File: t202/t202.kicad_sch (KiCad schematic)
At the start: 7 parts, among them J1 Conn_02x04_Counter_Clockwise, SW1 SW_Push, U1 ATtiny202-SS

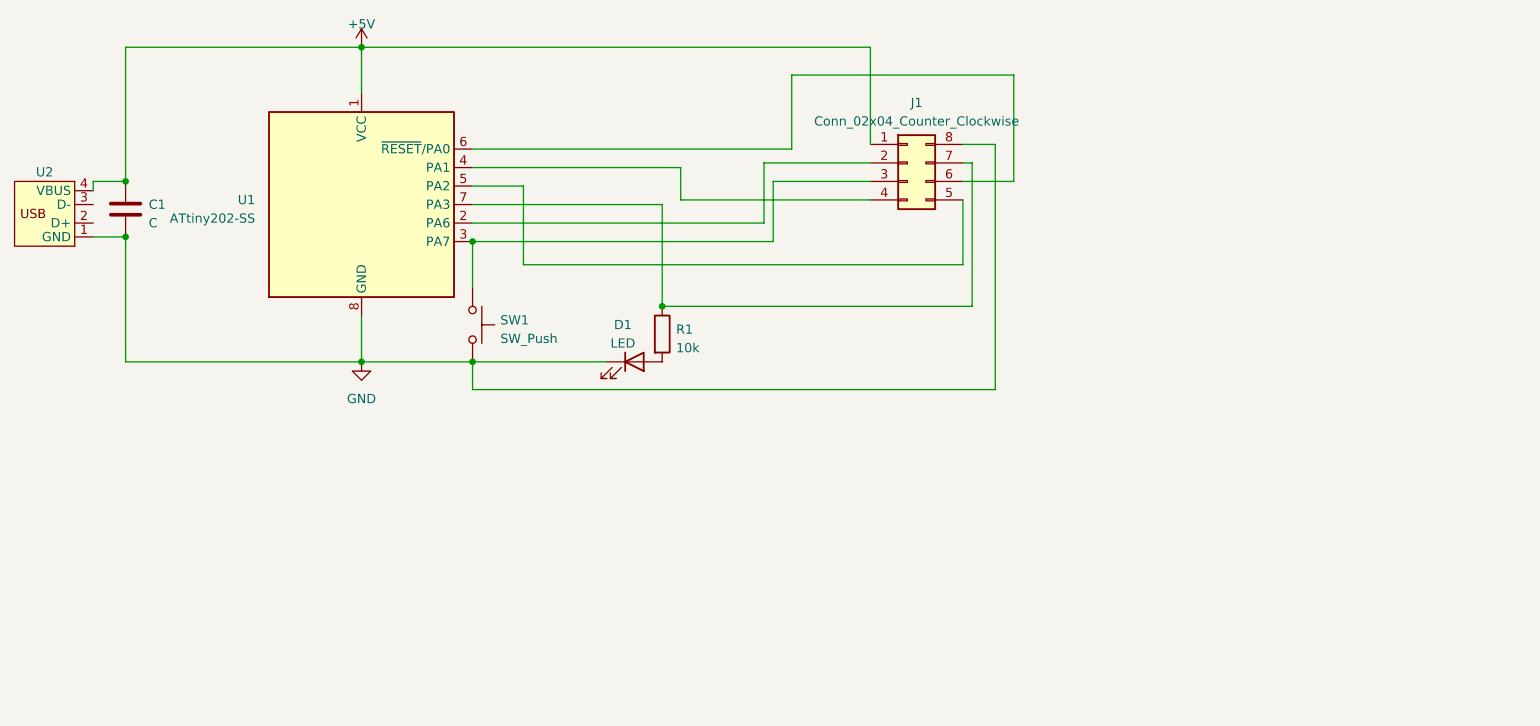
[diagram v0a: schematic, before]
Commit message: -
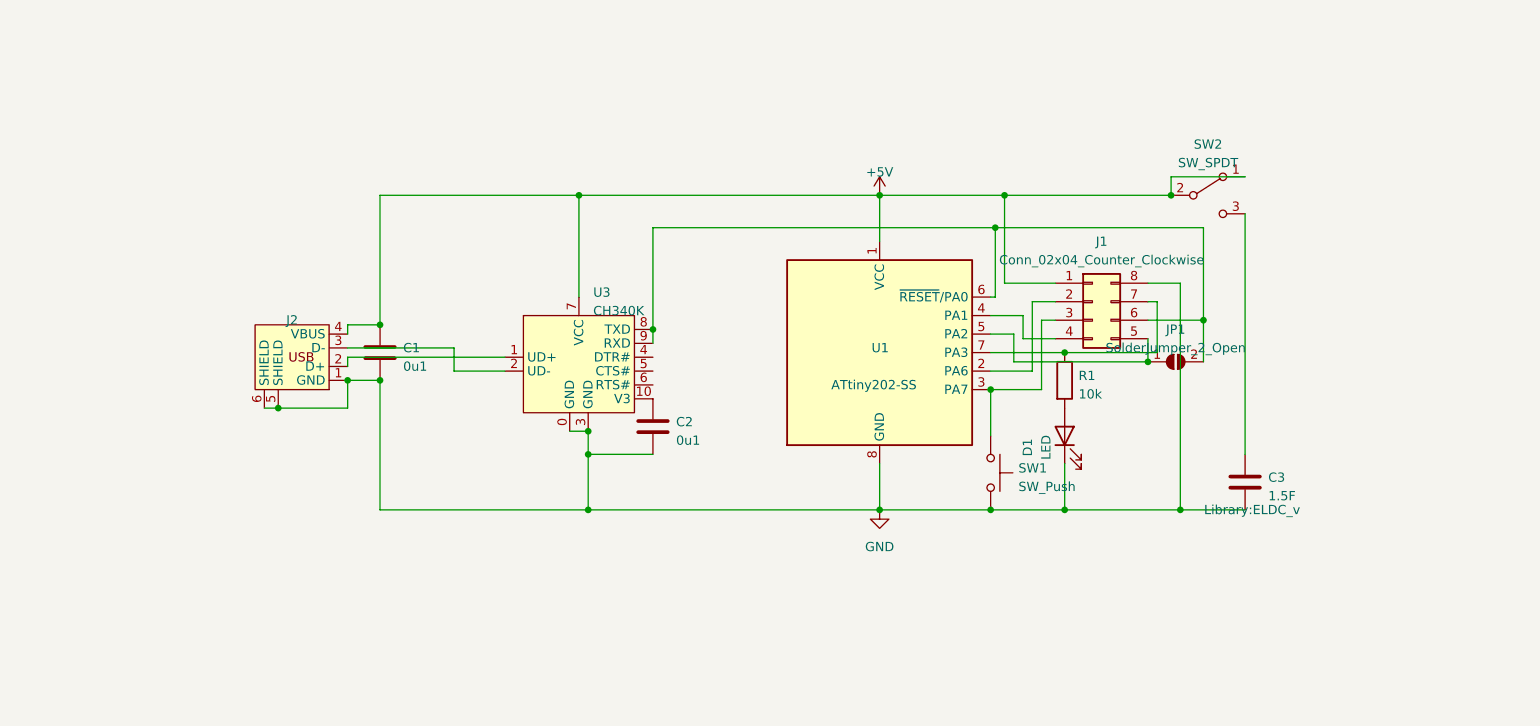
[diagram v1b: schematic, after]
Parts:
- removed U2: ~, Library:PCB_USB_Conn, symbol usb_a_pcb:PCB_USB_Conn
- added C2: 0u1, Capacitor_SMD:C_0603_1608Metric_Pad1.08x0.95mm_HandSolder, symbol Device:C
- added C3: 1.5F, Library:ELDC_v, symbol Device:C
- added J2: ~, Library:PCB_USB_Conn, symbol usb_a_pcb:PCB_USB_Conn
- added JP1: SolderJumper_2_Open, Library:sop_jumper, symbol Jumper:SolderJumper_2_Open
- added SW2: SW_SPDT, Library:3pad_2.5_h, symbol Switch:SW_SPDT
- added U3: CH340K, Package_SO:SSOP-10_3.9x4.9mm_P1.00mm, symbol akizuki:CH340K
- C1: value C -> 0u1
- SW1: footprint Library:THAF01-NC-R -> Library:TVAF06-A020B-R
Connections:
- net +5V: now also J2.4 (VBUS), SW2.1 (A), SW2.2 (B), U3.7 (VCC)
- net GND: now also C2.2, C3.2, J2.1 (GND), J2.5 (SHIELD), J2.6 (SHIELD), U3.0 (GND), U3.3 (GND)
- net at J1.5 (Pin_5), U1.5 (PA2): now also JP1.1 (A)
- net at J1.6 (Pin_6), U1.6 (~{RESET}/PA0): now also JP1.2 (B), U3.8 (TXD), U3.9 (RXD)
- new net: C2.1, U3.10 (V3)
- new net: C3.1, SW2.3 (C)
- new net: J2.2 (D+), U3.1 (UD+)
- new net: J2.3 (D-), U3.2 (UD-)
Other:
- moved on the sheet: C1, D1, J1, R1, SW1, U1

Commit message: -
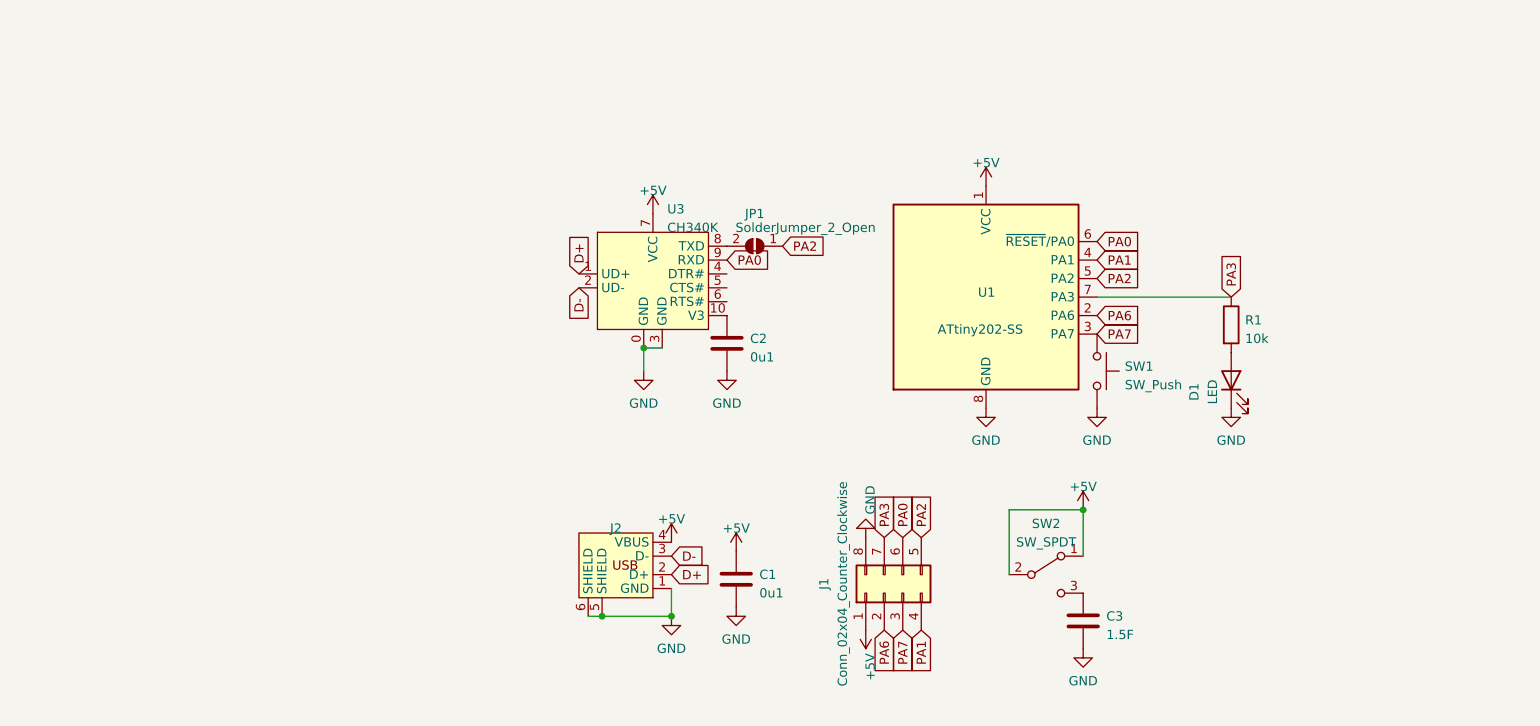
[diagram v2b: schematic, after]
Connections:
- net PA3: now reaches J1.7 (Pin_7), R1.1, U1.7 (PA3)
- net PA6: now reaches J1.2 (Pin_2), U1.2 (PA6)
- net PA7: now reaches J1.3 (Pin_3), SW1.1, U1.3 (PA7)
- net PA1: now reaches J1.4 (Pin_4), U1.4 (PA1)
- net PA2: now reaches J1.5 (Pin_5), JP1.1 (A), U1.5 (PA2)
- net PA0: now reaches J1.6 (Pin_6), U1.6 (~{RESET}/PA0), U3.9 (RXD)
- net PA0: no longer JP1.2 (B), U3.8 (TXD)
- net D+: now reaches J2.2 (D+), U3.1 (UD+)
- net D-: now reaches J2.3 (D-), U3.2 (UD-)
- new net: JP1.2 (B), U3.8 (TXD)
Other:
- moved on the sheet: C1, C2, C3, D1, J1, J2, JP1, R1, SW1, SW2, U1, U3

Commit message: -
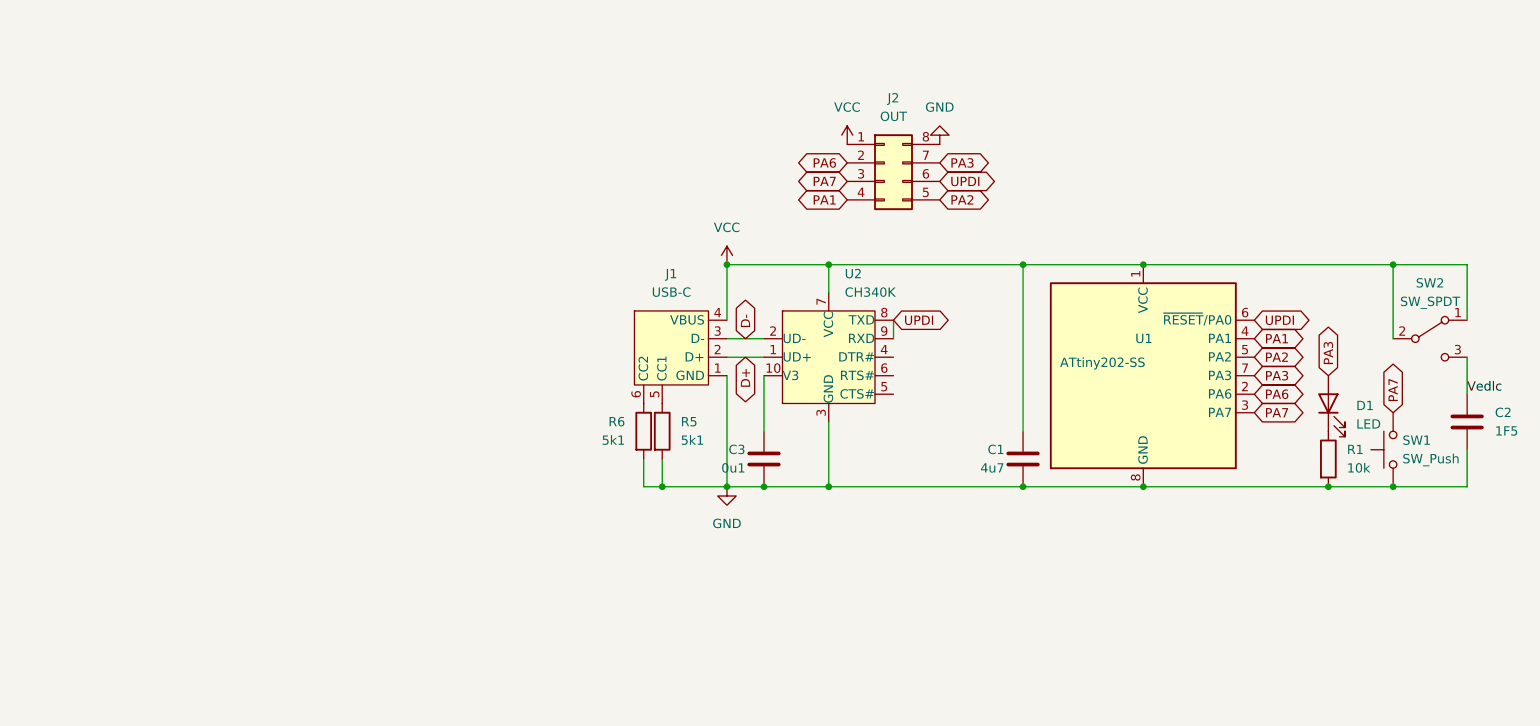
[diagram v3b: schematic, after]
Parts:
- removed J1: Conn_02x04_Counter_Clockwise, Package_DIP:DIP-8_W7.62mm, symbol Connector_Generic:Conn_02x04_Counter_Clockwise
- removed J2: ~, Library:PCB_USB_Conn, symbol usb_a_pcb:PCB_USB_Conn
- removed JP1: SolderJumper_2_Open, Library:sop_jumper, symbol Jumper:SolderJumper_2_Open
- removed U3: CH340K, Package_SO:SSOP-10_3.9x4.9mm_P1.00mm, symbol akizuki:CH340K
- added J1: USB-C, Library:USB-C, symbol Library:USB-C
- added J2: OUT, Package_DIP:DIP-8_W7.62mm_Socket, symbol Connector_Generic:Conn_02x04_Counter_Clockwise
- added R5, R6: 5k1, Resistor_SMD:R_0603_1608Metric, symbol Device:R
- added U2: CH340K, Package_SO:SSOP-10_3.9x4.9mm_P1.00mm, symbol Library:CH340K
- C1: value 0u1 -> 4u7; footprint Capacitor_SMD:C_0603_1608Metric_Pad1.08x0.95mm_HandSolder -> Capacitor_SMD:C_0603_1608Metric
- C2: value 0u1 -> 1F5; footprint Capacitor_SMD:C_0603_1608Metric_Pad1.08x0.95mm_HandSolder -> Library:edlc
- C3: value 1.5F -> 0u1; footprint Library:ELDC_v -> Capacitor_SMD:C_0603_1608Metric
- D1: footprint LED_SMD:LED_0603_1608Metric_Pad1.05x0.95mm_HandSolder -> LED_SMD:LED_0603_1608Metric
- R1: footprint Resistor_SMD:R_0603_1608Metric_Pad0.98x0.95mm_HandSolder -> Resistor_SMD:R_0603_1608Metric
- SW1: footprint Library:TVAF06-A020B-R -> Library:sw_push_smd
- SW2: footprint Library:3pad_2.5_h -> Library:sw
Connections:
- net D+: now also J1.2 (D+), U2.1 (UD+)
- net D-: now also J1.3 (D-), U2.2 (UD-)
- net GND: now also R1.2, SW1.1, J1.1 (GND), J2.8 (Pin_8), R5.2, R6.2, U2.3 (GND); no longer D1.1 (K), SW1.2
- net PA1: now also J2.4 (Pin_4)
- net PA2: now also J2.5 (Pin_5)
- net PA3: now also D1.2 (A), J2.7 (Pin_7); no longer R1.1
- net PA6: now also J2.2 (Pin_2)
- net PA7: now also SW1.2, J2.3 (Pin_3); no longer SW1.1
- net Vedlc: now reaches C2.1
- net Vedlc: now also SW2.3 (C)
- net at C3.1: now also U2.10 (V3); no longer SW2.3 (C)
- net +5V renamed VCC
- net VCC: now also J1.4 (VBUS), J2.1 (Pin_1), U2.7 (VCC)
- net PA0 renamed UPDI
- net UPDI: now also J2.6 (Pin_6), U2.8 (TXD), U2.9 (RXD)
- new net: D1.1 (K), R1.1
- new net: J1.6 (CC2), R6.1
- new net: J1.5 (CC1), R5.1
